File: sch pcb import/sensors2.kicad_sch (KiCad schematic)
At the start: 32 parts, among them J501 Conn_Coaxial, J502 0734120114, J503 0734120114, J504 Micro_SD_Card, J505 Screw_Terminal_01x06, U501 RFM98W-433S2, U502 NEO-6M-GPS, U503 W25Q128JVS

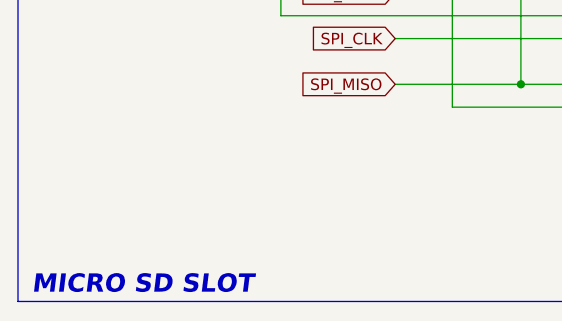
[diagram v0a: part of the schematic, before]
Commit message: minor changes
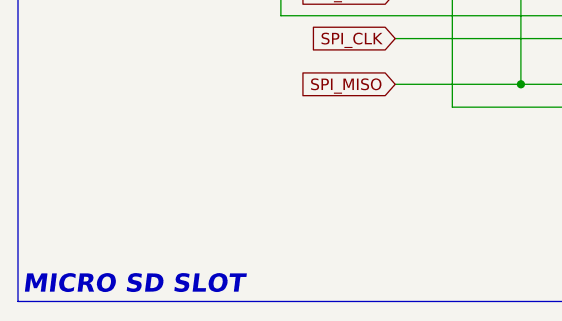
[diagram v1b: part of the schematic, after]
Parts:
- C501, C502, C503, C504, C505, C506, C507, C508, C509, C510, C511, C512: footprint (none) -> Capacitor_SMD:C_0603_1608Metric
- D501: footprint (none) -> LED_SMD:LED_0603_1608Metric
- L501, L502: footprint (none) -> Inductor_SMD:L_0402_1005Metric
- R501, R502, R503, R504, R505, R506, R507, R508, R509: footprint (none) -> Resistor_SMD:R_0603_1608Metric
- U501: footprint (none) -> RF_Module:HOPERF_RFM9XW_SMD
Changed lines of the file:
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@@
 	(text "MICRO SD SLOT\n"
 		(exclude_from_sim no)
-		(at 14.224 195.072 0)
+		(at 13.208 195.072 0)
 		(effects
 			(font
@@
 			)
 		)
-		(property "Footprint" ""
+		(property "Footprint" "Resistor_SMD:R_0603_1608Metric"
 			(at 82.55 71.628 90)
 			(effects
@@
 			)
 		)
-		(property "Footprint" ""
+		(property "Footprint" "Capacitor_SMD:C_0603_1608Metric"
 			(at 23.8252 29.21 0)
 			(effects
@@
 			)
 		)
-		(property "Footprint" ""
+		(property "Footprint" "Capacitor_SMD:C_0603_1608Metric"
 			(at 154.6352 27.94 0)
 			(effects
@@
 			)
 		)
-		(property "Footprint" ""
+		(property "Footprint" "Resistor_SMD:R_0603_1608Metric"
 			(at 77.978 148.59 90)
 			(effects
@@
 			)
 		)
-		(property "Footprint" ""
+		(property "Footprint" "Resistor_SMD:R_0603_1608Metric"
 			(at 70.358 148.59 90)
 			(effects
@@
 			)
 		)
-		(property "Footprint" ""
+		(property "Footprint" "Resistor_SMD:R_0603_1608Metric"
 			(at 100.838 148.59 90)
 			(effects
@@
 			)
 		)
-		(property "Footprint" ""
+		(property "Footprint" "Capacitor_SMD:C_0603_1608Metric"
 			(at 268.9352 144.78 0)
 			(effects
@@
 			)
 		)
-		(property "Footprint" ""
+		(property "Footprint" "RF_Module:HOPERF_RFM9XW_SMD"
 			(at 146.05 21.59 0)
 			(effects
@@
 			)
 		)
-		(property "Footprint" ""
+		(property "Footprint" "Inductor_SMD:L_0402_1005Metric"
 			(at 76.2 25.4 0)
 			(effects
@@
 			)
 		)
-		(property "Footprint" ""
+		(property "Footprint" "Capacitor_SMD:C_0603_1608Metric"
 			(at 147.0152 27.94 0)
 			(effects
@@
 			)
 		)
-		(property "Footprint" ""
+		(property "Footprint" "Resistor_SMD:R_0603_1608Metric"
 			(at 93.218 148.59 90)
 			(effects
@@
 			)
 		)
-		(property "Footprint" ""
+		(property "Footprint" "Capacitor_SMD:C_0603_1608Metric"
 			(at 225.7552 31.75 0)
 			(effects
@@
 			)
 		)
-		(property "Footprint" ""
+		(property "Footprint" "Capacitor_SMD:C_0603_1608Metric"
 			(at 21.2852 146.05 0)
 			(effects
@@
 			)
 		)
-		(property "Footprint" ""
+		(property "Footprint" "Resistor_SMD:R_0603_1608Metric"
 			(at 206.248 130.81 90)
 			(effects
@@
 			)
 		)
-		(property "Footprint" ""
+		(property "Footprint" "Resistor_SMD:R_0603_1608Metric"
 			(at 62.738 148.59 90)
 			(effects
@@
 			)
 		)
-		(property "Footprint" ""
+		(property "Footprint" "Inductor_SMD:L_0402_1005Metric"
 			(at 234.95 21.59 0)
 			(effects
@@
 			)
 		)
-		(property "Footprint" ""
+		(property "Footprint" "Capacitor_SMD:C_0603_1608Metric"
 			(at 31.4452 29.21 0)
 			(effects
@@
 			)
 		)
-		(property "Footprint" ""
+		(property "Footprint" "Resistor_SMD:R_0603_1608Metric"
 			(at 85.598 148.59 90)
 			(effects
@@
 			)
 		)
-		(property "Footprint" ""
+		(property "Footprint" "Resistor_SMD:R_0603_1608Metric"
 			(at 57.15 27.178 90)
 			(effects
@@
 			)
 		)
-		(property "Footprint" ""
+		(property "Footprint" "Capacitor_SMD:C_0603_1608Metric"
 			(at 268.9352 68.58 0)
 			(effects
@@
 			)
 		)
-		(property "Footprint" ""
+		(property "Footprint" "Capacitor_SMD:C_0603_1608Metric"
 			(at 276.5552 68.58 0)
 			(effects
@@
 			)
 		)
-		(property "Footprint" ""
+		(property "Footprint" "Capacitor_SMD:C_0603_1608Metric"
 			(at 28.9052 146.05 0)
 			(effects
@@
 			)
 		)
-		(property "Footprint" ""
+		(property "Footprint" "Capacitor_SMD:C_0603_1608Metric"
 			(at 261.3152 144.78 0)
 			(effects
@@
 			)
 		)
-		(property "Footprint" ""
+		(property "Footprint" "Capacitor_SMD:C_0603_1608Metric"
 			(at 244.8052 31.75 0)
 			(effects
@@
 			)
 		)
-		(property "Footprint" ""
+		(property "Footprint" "LED_SMD:LED_0603_1608Metric"
 			(at 92.71 78.74 0)
 			(effects
